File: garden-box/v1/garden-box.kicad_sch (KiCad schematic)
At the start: 22 parts, among them J1 Conn_01x02_Male, J10 Screw_Terminal_01x02, J11 Screw_Terminal_01x02, J12 Conn_01x06_Male, J13 Conn_01x06_Male, J2 Conn_01x03_Male, J3 Conn_01x04_Male, J4 Screw_Terminal_01x02, J5 Screw_Terminal_01x02, J6 Screw_Terminal_01x02, J7 Screw_Terminal_01x02, J8 Screw_Terminal_01x02, J9 Screw_Terminal_01x02, SW1 SW_Push_DPDT, SW2 SW_Push_DPDT, SW3 SW_Push_DPDT, SW4 SW_Push_DPDT, SW5 SW_Push_DPDT, SW6 SW_Push_DPDT, T1 Transformer_1P_2S, U1 LM7805_TO220, U2 ESP32-POE-ISO

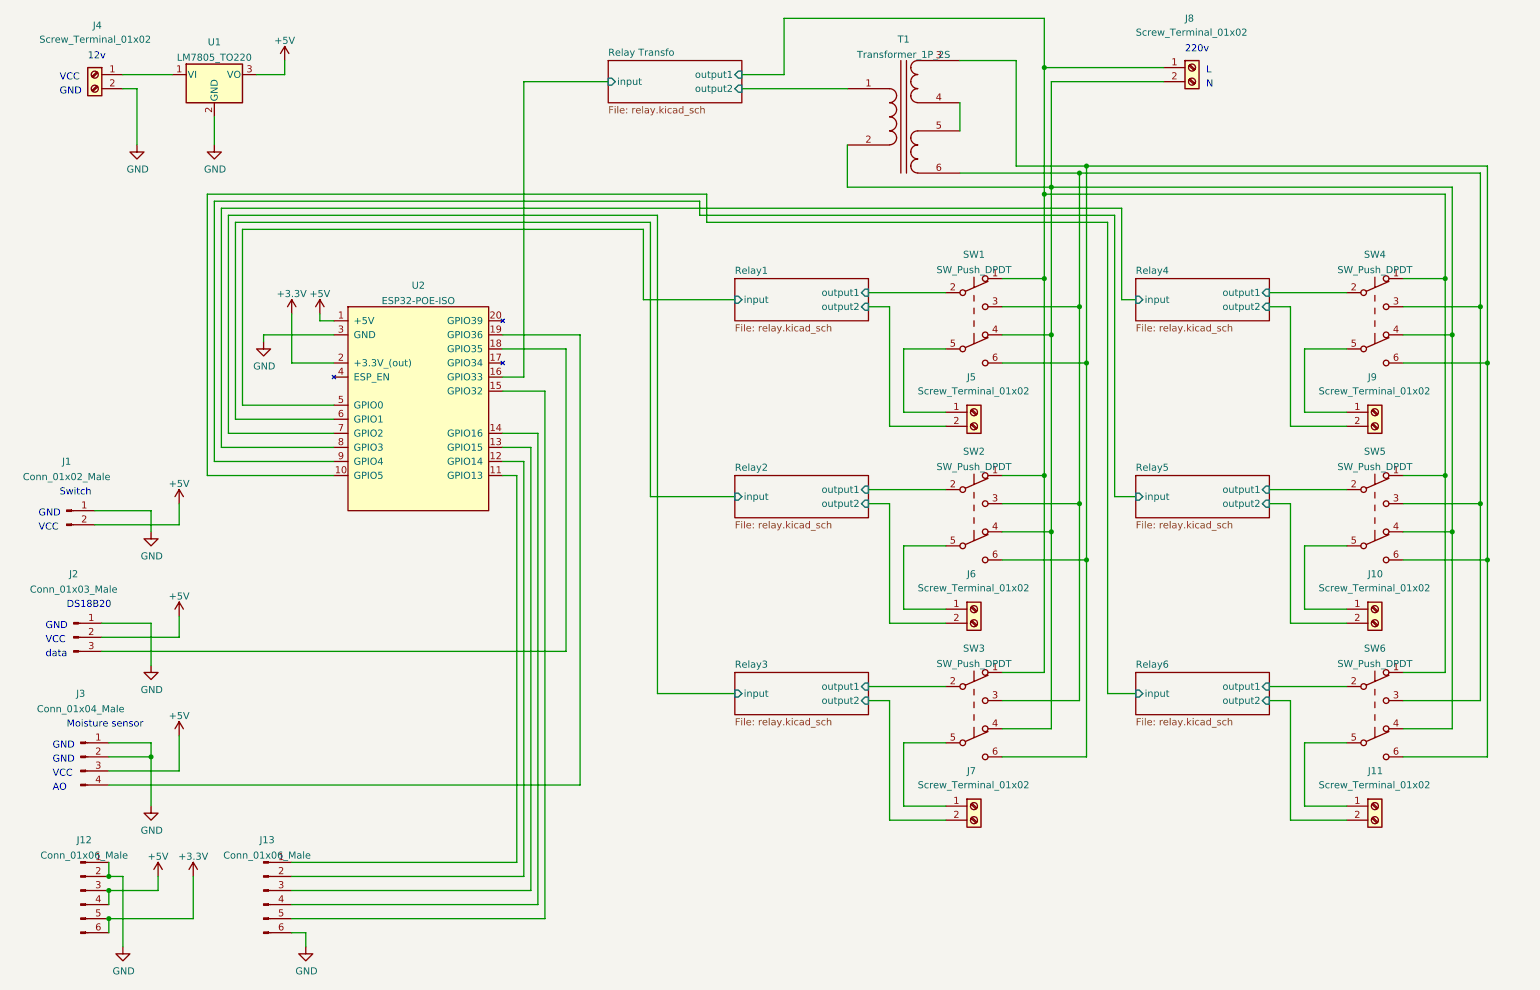
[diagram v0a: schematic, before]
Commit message: init new v1
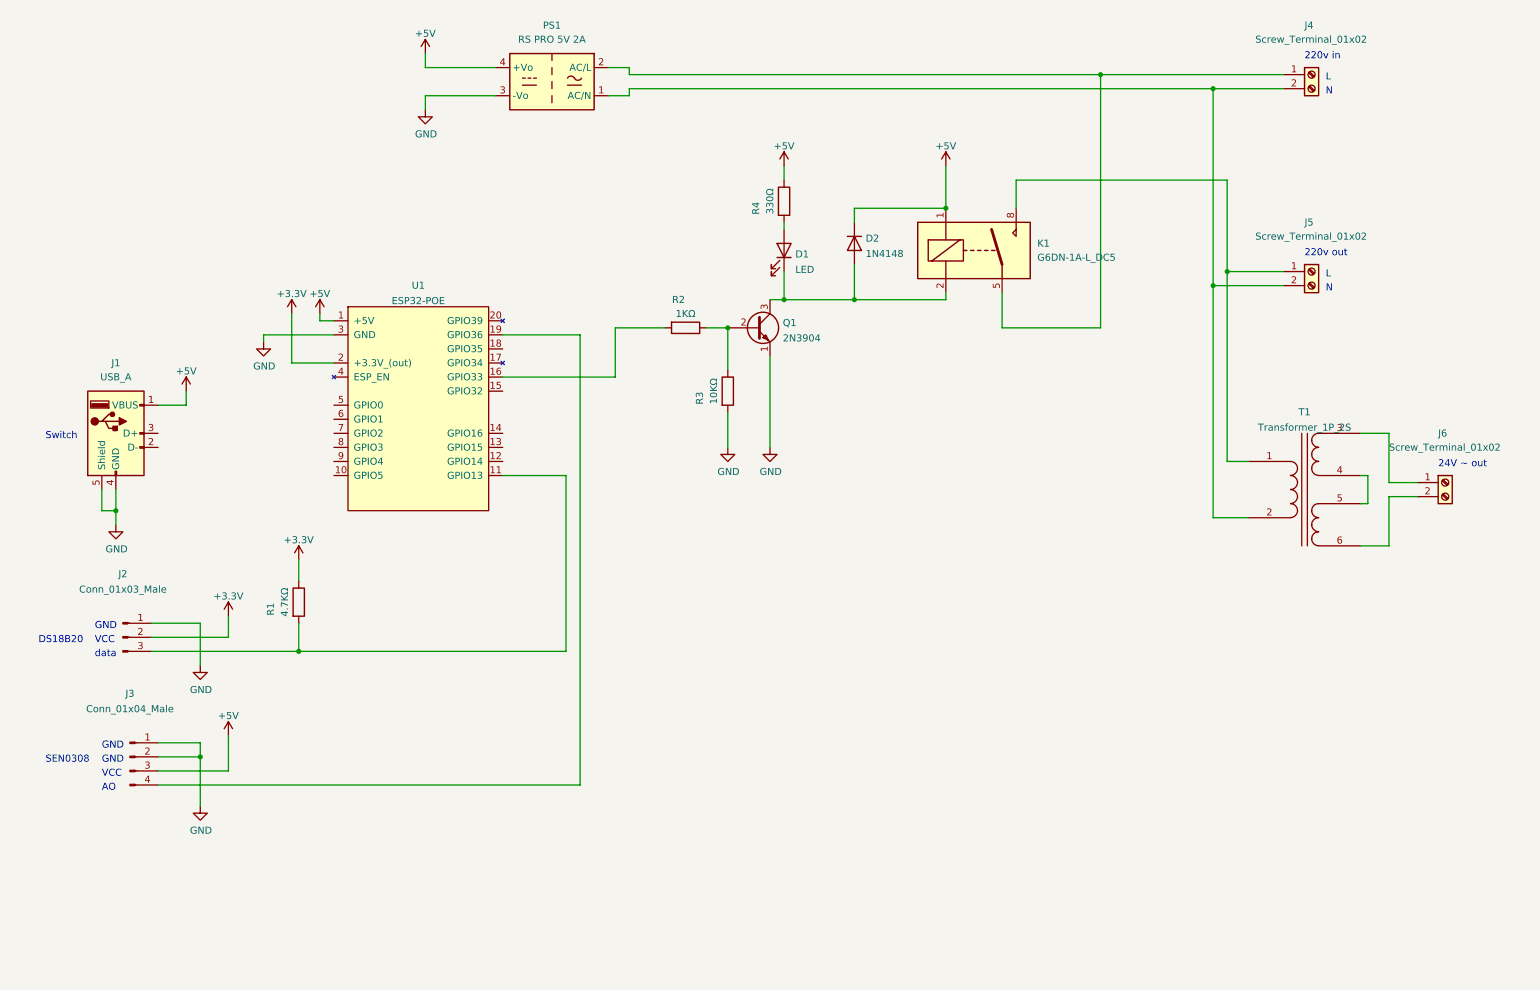
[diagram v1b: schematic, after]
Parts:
- removed J1: Conn_01x02_Male, Connector_PinHeader_2.54mm:PinHeader_1x02_P2.54mm_Vertical, symbol Connector:Conn_01x02_Male
- removed J10, J11, J7, J8, J9: Screw_Terminal_01x02, TerminalBlock:TerminalBlock_bornier-2_P5.08mm, symbol Connector:Screw_Terminal_01x02
- removed J12, J13: Conn_01x06_Male, Connector_PinHeader_2.54mm:PinHeader_1x06_P2.54mm_Vertical, symbol Connector:Conn_01x06_Male
- removed SW1, SW2, SW3, SW4, SW5, SW6: SW_Push_DPDT, symbol Switch:SW_Push_DPDT
- removed U1: LM7805_TO220, Package_TO_SOT_THT:TO-220-3_Vertical, symbol Regulator_Linear:LM7805_TO220
- added D1: LED, Diode_SMD:D_0805_2012Metric, symbol Device:LED
- added D2: 1N4148, Diode_SMD:D_SOD-123, symbol Diode:1N4148
- added J1: USB_A, rs-online:875200010BLF, symbol Connector:USB_A
- added K1: G6DN-1A-L_DC5, rs-online:G6DN-1A-L, symbol mylife-symbols:G6DN-1A-L_DC5
- added PS1: RS PRO 5V 2A, mylife-footprints:RS PRO 5V 2A, symbol Converter_ACDC:IRM-10-5
- added Q1: 2N3904, jlcpcb:SOT-23-3_L2.9-W1.3-P1.90-LS2.4-TR, symbol Transistor_BJT:2N3904
- added R1: 4.7KΩ, Resistor_SMD:R_0402_1005Metric, symbol Device:R
- added R2: 1KΩ, Resistor_SMD:R_0402_1005Metric, symbol Device:R
- added R3: 10KΩ, Resistor_SMD:R_0402_1005Metric, symbol Device:R
- added R4: 330Ω, Resistor_SMD:R_0402_1005Metric, symbol Device:R
- T1: footprint (none) -> rs-online:VCM36212
- U1: renamed from U2; value ESP32-POE-ISO -> ESP32-POE; footprint (none) -> mylife-footprints:ESP32-POE
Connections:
- net Relay Transfo/output2 is gone; now on an unnamed net: T1.1 (AA)
- net Relay1/output2 is gone; now on an unnamed net: J5.2 (Pin_2)
- net Relay2/output2 is gone; now on an unnamed net: J6.2 (Pin_2)
- net +3V3: now also J2.2 (Pin_2), R1.1
- net +5V: now also D2.1 (K), J1.1 (VBUS), K1.1, PS1.4 (+Vo), R4.1; no longer J2.2 (Pin_2)
- net GND: now also J1.4 (GND), J1.5 (Shield), PS1.3 (-Vo), Q1.1 (E), R3.2; no longer J4.2 (Pin_2)
- net at J6.1 (Pin_1): now also T1.3 (SA)
- net at T1.2 (AB): now also J4.2 (Pin_2), PS1.1 (AC/N)
- net at J5.1 (Pin_1): now also K1.8
- net at U1.11 (GPIO13): now also J2.3 (Pin_3), R1.2
- net at J4.1 (Pin_1): now also K1.5, PS1.2 (AC/L)
- net at U1.18 (GPIO35): no longer J2.3 (Pin_3)
- net Relay Transfo/input: no longer names the net of U1.16 (GPIO33)
- net Relay Transfo/input: now also R2.2
- net Relay1/input: no longer names the net of U1.5 (GPIO0)
- net Relay2/input: no longer names the net of U1.6 (GPIO1)
- net Relay3/input: no longer names the net of U1.7 (GPIO2)
- net Relay4/input: no longer names the net of U1.8 (GPIO3)
- net Relay5/input: no longer names the net of U1.9 (GPIO4)
- net Relay6/input: no longer names the net of U1.10 (GPIO5)
- new net: Q1.2 (B), R2.1, R3.1
- new net: D1.1 (K), D2.2 (A), K1.2, Q1.3 (C)
- new net: D1.2 (A), R4.2
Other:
- removed sheet Relay Transfo
- removed sheet Relay1
- removed sheet Relay2
- removed sheet Relay3
- removed sheet Relay4
- removed sheet Relay5
- removed sheet Relay6
- note added: "220v in"
- note added: "220v out"
- note added: "24V ~ out"
- note added: "SEN0308"
- note removed: "12v"
- note removed: "220v"
- note removed: "Moisture sensor"
- moved on the sheet: J2, J3
